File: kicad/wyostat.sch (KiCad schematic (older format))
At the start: 71 parts, among them J1 PWR_In, J10 MOSI, J11 RST, J12 GND, J13 AC_IN, J14 ~RST, J2 OUT1, J3 OUT2, J4 I2C_ext1, J5 MISO, J6 3V3, J7 OUT3, J8 SCK, J9 SPI, Q1 BT136-600, Q2 BT136-600, Q3 BT136-600, U1 MOC3063M, U2 Wemos-Lolin, U3 MOC3063M, U4 MOC3063M, U5 MAX17502FATB+T

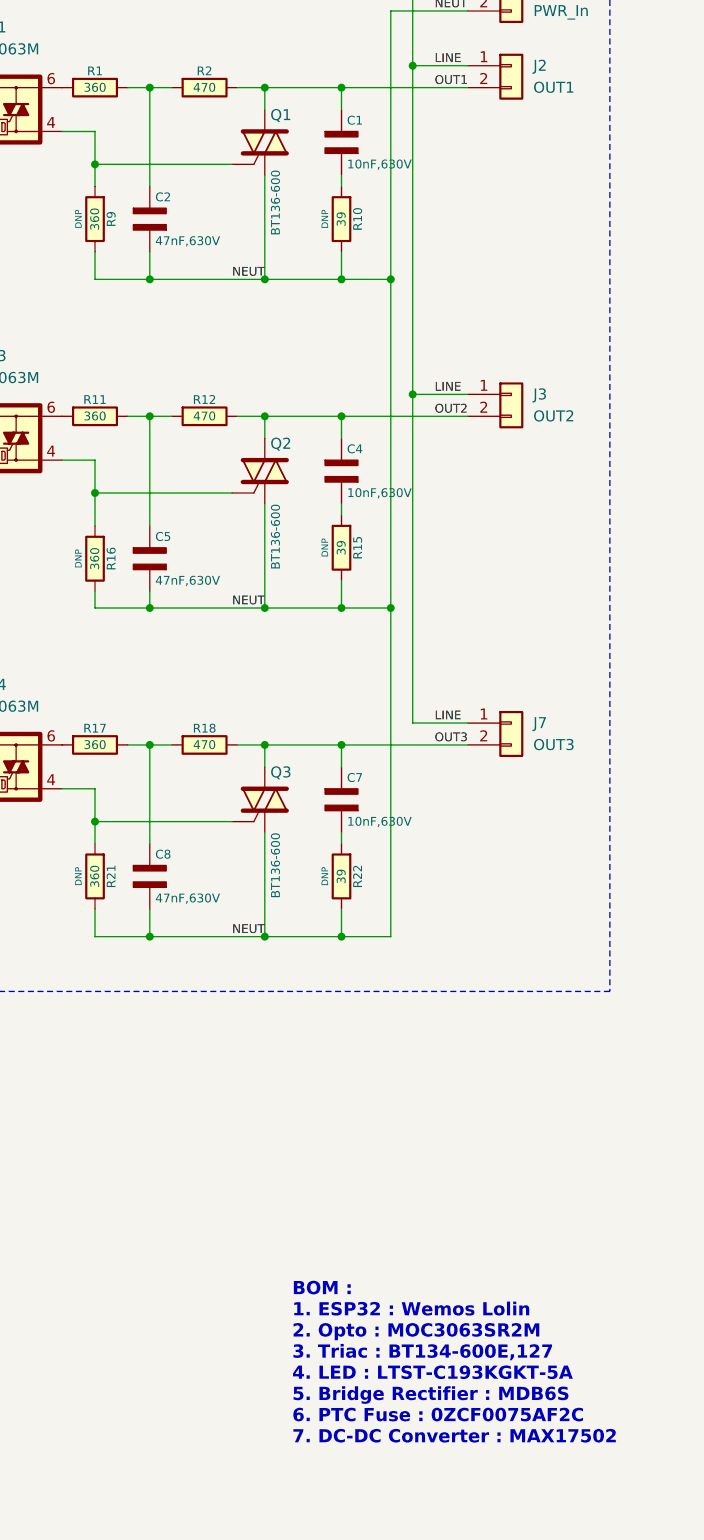
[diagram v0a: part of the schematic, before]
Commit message: kicad schematic, WIP
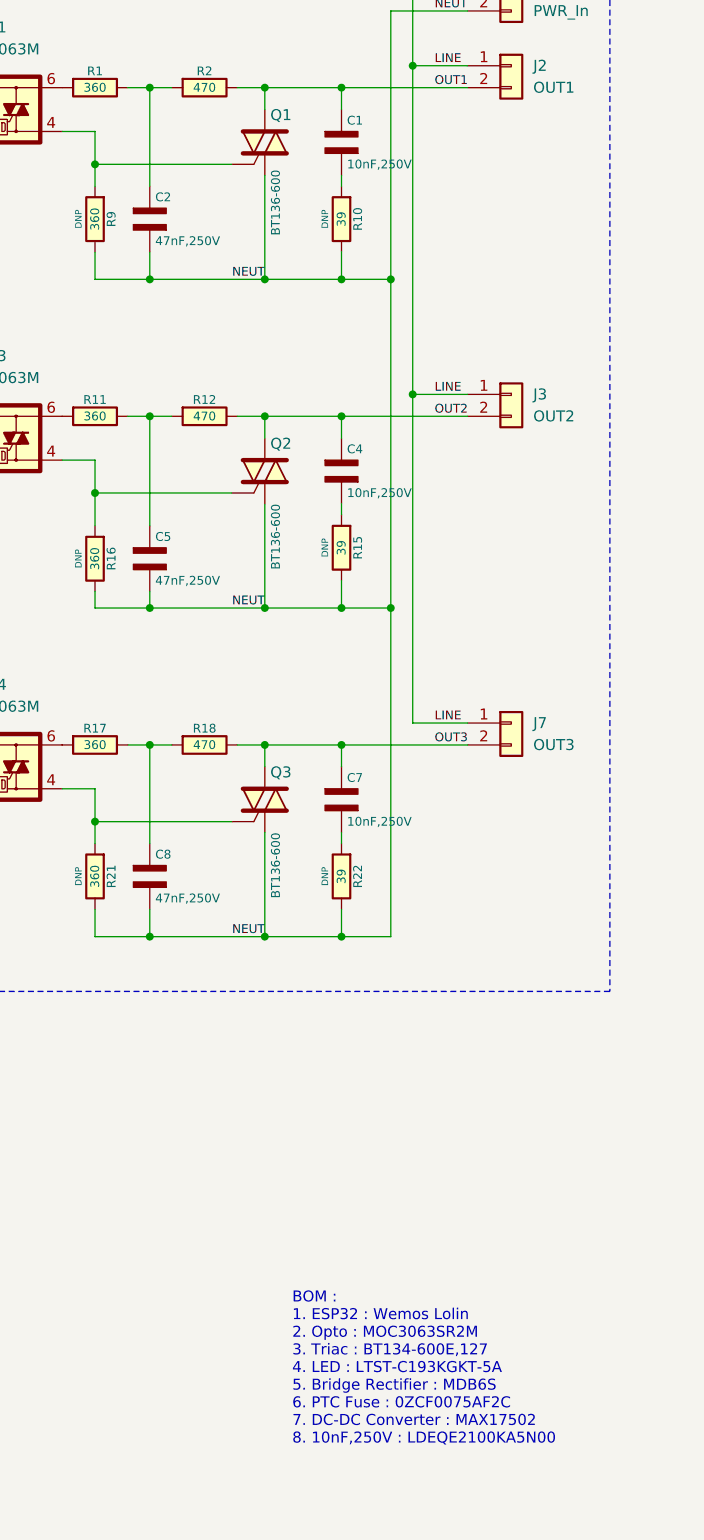
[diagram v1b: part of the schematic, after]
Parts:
- C1: value 10nF,630V -> 10nF,250V; footprint (none) -> Capacitors_Tantalum_SMD:CP_Tantalum_Case-E_EIA-7260-38_Hand
- C11, C12, C13, C14, C9: footprint (none) -> Capacitors_SMD:C_0805
- C2, C5, C8: value 47nF,630V -> 47nF,250V
- C3, C6: footprint KlokTHREEjr_libs:c_0805 -> Capacitors_SMD:C_0805
- C4, C7: value 10nF,630V -> 10nF,250V
- D1, D2, D3: footprint (none) -> LEDs:LED_0603
- F1: footprint (none) -> Fuse_Holders_and_Fuses:Fuse_SMD2920
- J1, J13, J2, J3, J7: footprint (none) -> Connectors_Terminal_Blocks:TerminalBlock_Pheonix_MPT-2.54mm_2pol
- J10, J11, J12, J5, J6, J8: footprint KlokTHREEjr_libs:BreakOutPad -> Pin_Headers:Pin_Header_Straight_1x01
- J14: footprint (none) -> Pin_Headers:Pin_Header_Straight_1x01
- J4: footprint KlokTHREEjr_libs:Header_4x1 -> Pin_Headers:Pin_Header_Straight_1x04
- J9: footprint KlokTHREEjr_libs:Header_ISP -> Pin_Headers:Pin_Header_Straight_2x03
- JP1, JP2, JP3: footprint (none) -> LEDs:LED_0402
- R1, R10, R11, R12, R13, R14, R15, R16, R17, R18, R19, R2, R20, R21, R22, R3, R4, R9: footprint (none) -> Resistors_SMD:R_0805
- R5, R6, R7, R8: footprint KlokTHREEjr_libs:r_0805 -> Resistors_SMD:R_0805
- U1, U3, U4: footprint (none) -> Opto-Devices:Optocoupler_6pin_wide_Stile-I
- U5: footprint TDFN 10 -> (none)
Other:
- note added: "BOM :\n1. ESP32 : Wemos Lolin\n2. Opto : MOC3063SR2M\n3. Triac : BT134-600E,127\n4. LED : LTST-C193KGKT-5A\n5. Bridge Rectifier : MDB6S\n6. PTC Fuse : 0ZCF0075AF2C\n7. DC-DC Converter : MAX17502\n8. 10nF,250V : LDEQE2100KA5N00"
- note removed: "BOM :\n1. ESP32 : Wemos Lolin\n2. Opto : MOC3063SR2M\n3. Triac : BT134-600E,127\n4. LED : LTST-C193KGKT-5A\n5. Bridge Rectifier : MDB6S\n6. PTC Fuse : 0ZCF0075AF2C\n7. DC-DC Converter : MAX17502"
